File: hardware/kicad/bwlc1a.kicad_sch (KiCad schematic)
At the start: 0 parts

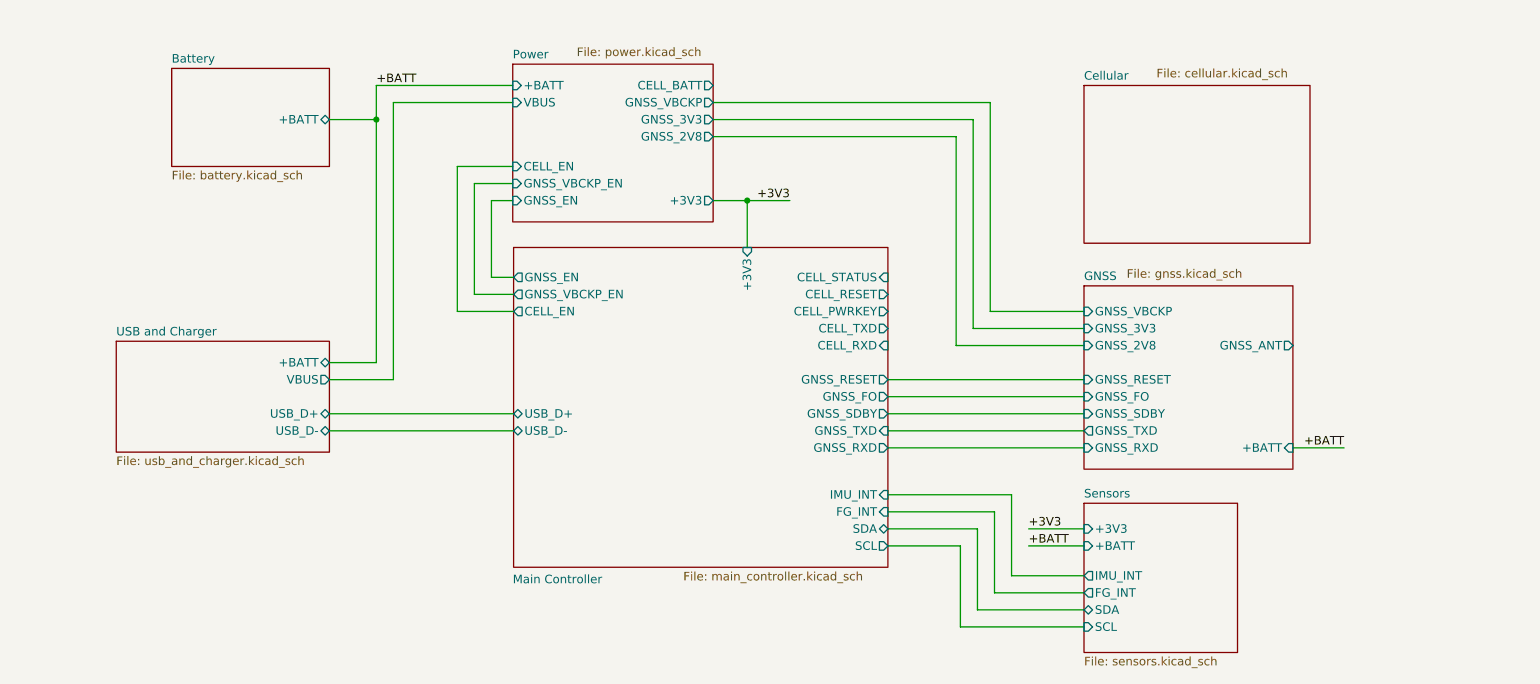
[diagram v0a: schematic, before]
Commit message: wip: revision 2
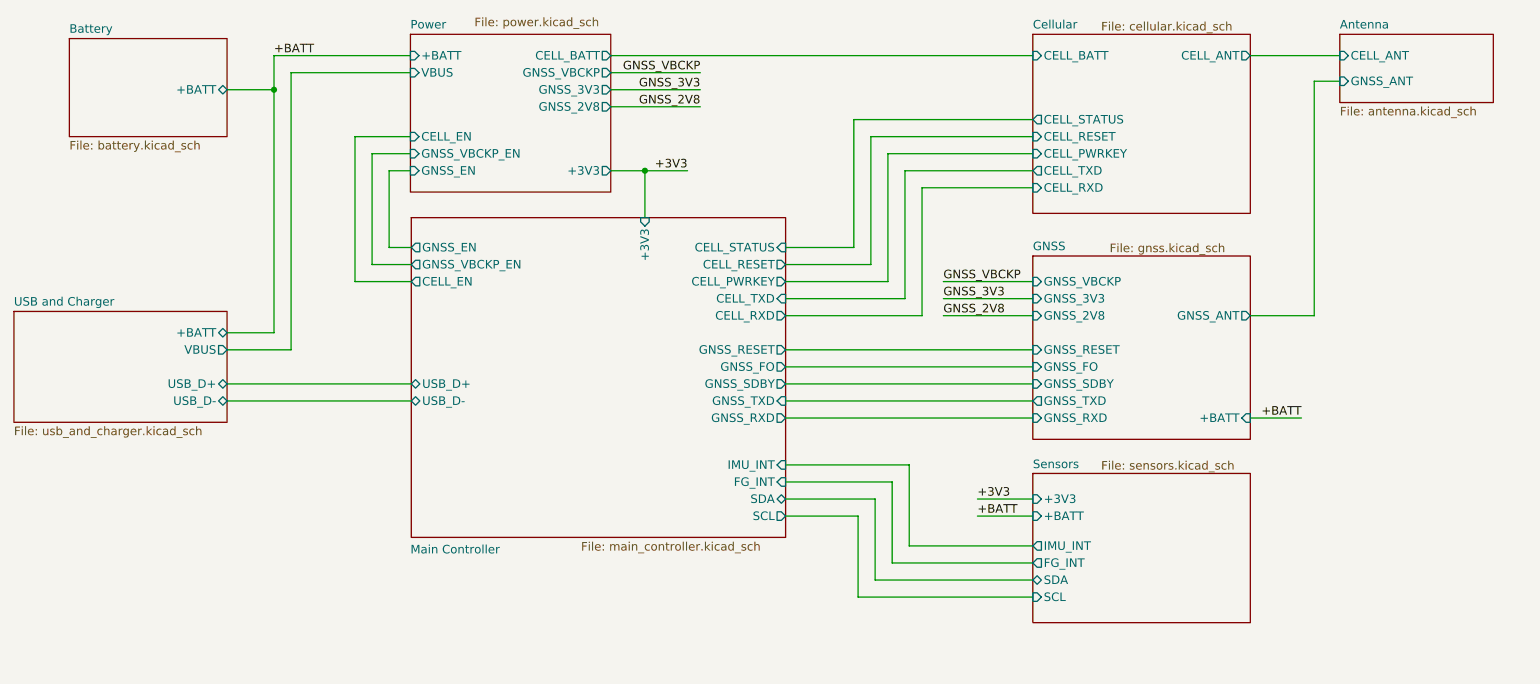
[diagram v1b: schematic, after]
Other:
- added sheet Antenna (antenna.kicad_sch)
- sheet Cellular ports: added CELL_ANT, CELL_BATT, CELL_PWRKEY, CELL_RESET, CELL_RXD, CELL_STATUS, CELL_TXD; removed none
